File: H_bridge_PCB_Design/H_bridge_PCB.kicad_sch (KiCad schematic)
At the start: 7 parts, among them U1 ESP32-WROOM-32

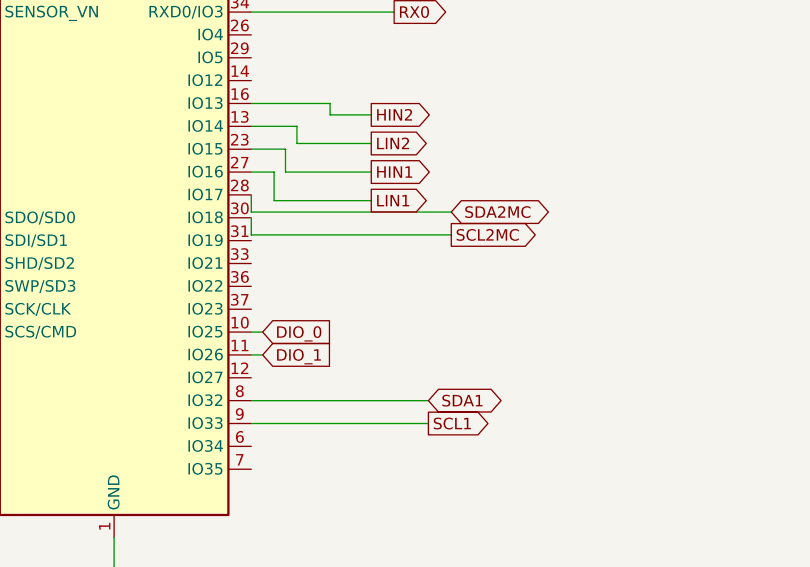
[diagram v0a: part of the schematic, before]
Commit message: huge changes output measurement
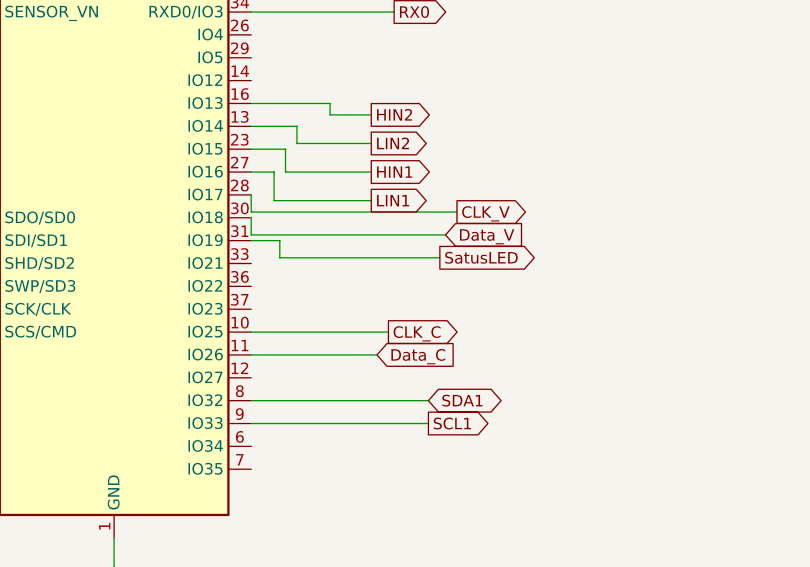
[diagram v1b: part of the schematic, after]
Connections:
- net SatusLED: now reaches U1.31 (IO19)
- net DIO_0 renamed CLK_C
- net DIO_1 renamed Data_C
- net SCL2MC renamed Data_V
- net SDA2MC renamed CLK_V
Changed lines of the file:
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@@
-	(wire
-		(pts
-			(xy 198.12 229.235) (xy 199.39 229.235)
-		)
-		(stroke
-			(width 0)
-			(type default)
-		)
-	)
 	(wire
 		(pts
@@
 	(wire
 		(pts
-			(xy 198.12 213.36) (xy 220.345 213.36)
-		)
-		(stroke
-			(width 0)
-			(type default)
-		)
-	)
-	(wire
-		(pts
 			(xy 201.93 208.915) (xy 211.455 208.915)
 		)
@@
 	(wire
 		(pts
+			(xy 201.295 216.535) (xy 198.12 216.535)
+		)
+		(stroke
+			(width 0)
+			(type default)
+		)
+	)
+	(wire
+		(pts
 			(xy 207.645 179.705) (xy 207.645 183.515)
 		)
@@
 	(wire
 		(pts
-			(xy 198.12 226.695) (xy 199.39 226.695)
-		)
-		(stroke
-			(width 0)
-			(type default)
-		)
-	)
-	(wire
-		(pts
-			(xy 220.345 215.9) (xy 198.12 215.9)
+			(xy 198.12 213.36) (xy 198.12 211.455)
+		)
+		(stroke
+			(width 0)
+			(type default)
+		)
+	)
+	(wire
+		(pts
+			(xy 198.12 213.36) (xy 220.98 213.36)
 		)
 		(stroke
@@
 	(wire
 		(pts
+			(xy 198.12 215.9) (xy 219.71 215.9)
+		)
+		(stroke
+			(width 0)
+			(type default)
+		)
+	)
+	(wire
+		(pts
 			(xy 171.45 163.83) (xy 182.88 163.83)
 		)
@@
 	(wire
 		(pts
-			(xy 198.12 213.36) (xy 198.12 211.455)
+			(xy 213.36 226.695) (xy 198.12 226.695)
 		)
 		(stroke
@@
 	(wire
 		(pts
+			(xy 212.09 229.235) (xy 198.12 229.235)
+		)
+		(stroke
+			(width 0)
+			(type default)
+		)
+	)
+	(wire
+		(pts
 			(xy 201.93 206.375) (xy 198.12 206.375)
 		)
@@
 	(wire
 		(pts
+			(xy 201.295 218.44) (xy 201.295 216.535)
+		)
+		(stroke
+			(width 0)
+			(type default)
+		)
+	)
+	(wire
+		(pts
 			(xy 148.59 175.26) (xy 148.59 183.515)
 		)
@@
 		)
 	)
+	(wire
+		(pts
+			(xy 219.075 218.44) (xy 201.295 218.44)
+		)
+		(stroke
+			(width 0)
+			(type default)
+		)
+	)
 	(global_label "LIN1"
 		(shape output)
@@
 		(property "Intersheetrefs" "${INTERSHEET_REFS}"
 			(at 218.6131 212.09 0)
-			(effects
-				(font
-					(size 1.27 1.27)
-				)
-				(justify left)
-				(hide yes)
-			)
-		)
-	)
-	(global_label "DIO_1"
-		(shape input)
-		(at 199.39 229.235 0)
-		(fields_autoplaced yes)
-		(effects
-			(font
-				(size 1.27 1.27)
-			)
-			(justify left)
-		)
-		(property "Intersheetrefs" "${INTERSHEET_REFS}"
-			(at 207.7576 229.235 0)
 			(effects
 				(font
@@
 		)
 	)
-	(global_label "DIO_0"
-		(shape input)
-		(at 199.39 226.695 0)
-		(fields_autoplaced yes)
-		(effects
-			(font
-				(size 1.27 1.27)
-			)
-			(justify left)
-		)
-		(property "Intersheetrefs" "${INTERSHEET_REFS}"
-			(at 207.7576 226.695 0)
+	(global_label "CLK_V"
+		(shape output)
+		(at 220.98 213.36 0)
+		(fields_autoplaced yes)
+		(effects
+			(font
+				(size 1.27 1.27)
+			)
+			(justify left)
+		)
+		(property "Intersheetrefs" "${INTERSHEET_REFS}"
+			(at 229.5895 213.36 0)
 			(effects
 				(font
@@
 		)
 	)
-	(global_label "SCL2MC"
-		(shape output)
-		(at 220.345 215.9 0)
-		(fields_autoplaced yes)
-		(effects
-			(font
-				(size 1.27 1.27)
-			)
-			(justify left)
-		)
-		(property "Intersheetrefs" "${INTERSHEET_REFS}"
-			(at 230.7687 215.9 0)
-			(effects
-				(font
-					(size 1.27 1.27)
-				)
-				(justify left)
-				(hide yes)
-			)
-		)
-	)
-	(global_label "SDA2MC"
-		(shape bidirectional)
-		(at 220.345 213.36 0)
-		(fields_autoplaced yes)
-		(effects
-			(font
-				(size 1.27 1.27)
-			)
-			(justify left)
-		)
-		(property "Intersheetrefs" "${INTERSHEET_REFS}"
-			(at 231.9405 213.36 0)
-			(effects
-				(font
-					(size 1.27 1.27)
-				)
-				(justify left)
-				(hide yes)
-			)
-		)
-	)
 	(global_label "SCL1"
 		(shape output)
@@
 		)
 	)
+	(global_label "Data_V"
+		(shape input)
+		(at 219.71 215.9 0)
+		(fields_autoplaced yes)
+		(effects
+			(font
+				(size 1.27 1.27)
+			)
+			(justify left)
+		)
+		(property "Intersheetrefs" "${INTERSHEET_REFS}"
+			(at 229.0451 215.9 0)
+			(effects
+				(font
+					(size 1.27 1.27)
+				)
+				(justify left)
+				(hide yes)
+			)
+		)
+	)
 	(global_label "RX0"
 		(shape output)
@@
 		(property "Intersheetrefs" "${INTERSHEET_REFS}"
 			(at 220.6692 191.135 0)
+			(effects
+				(font
+					(size 1.27 1.27)
+				)
+				(justify left)
+				(hide yes)
+			)
+		)
+	)
+	(global_label "Data_C"
+		(shape input)
+		(at 212.09 229.235 0)
+		(fields_autoplaced yes)
+		(effects
+			(font
+				(size 1.27 1.27)
+			)
+			(justify left)
+		)
+		(property "Intersheetrefs" "${INTERSHEET_REFS}"
+			(at 221.6065 229.235 0)
+			(effects
+				(font
+					(size 1.27 1.27)
+				)
+				(justify left)
+				(hide yes)
+			)
+		)
+	)
+	(global_label "CLK_C"
+		(shape output)
+		(at 213.36 226.695 0)
+		(fields_autoplaced yes)
+		(effects
+			(font
+				(size 1.27 1.27)
+			)
+			(justify left)
+		)
+		(property "Intersheetrefs" "${INTERSHEET_REFS}"
+			(at 222.1509 226.695 0)
 			(effects
 				(font
@@
 			(effects
 				(font
+					(size 1.27 1.27)
+				)
+				(justify left)
+				(hide yes)
+			)
+		)
+	)
+	(global_label "SatusLED"
+		(shape output)
+		(at 219.075 218.44 0)
+		(fields_autoplaced yes)
+		(effects
+			(font
+				(size 1.27 1.27)
+			)
+			(justify left)
+		)
+		(property "Intersheetrefs" "${INTERSHEET_REFS}"
+			(at 230.7686 218.44 0)
+			(effects
+				(font

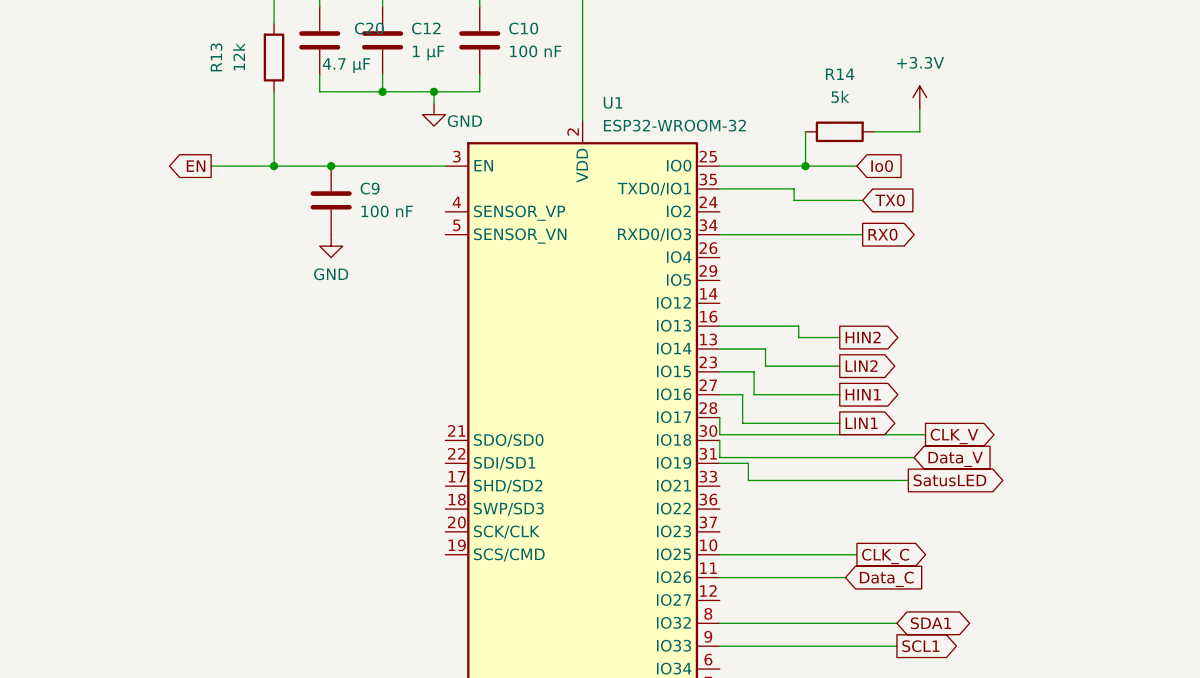
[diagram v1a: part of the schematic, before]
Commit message: new pcb
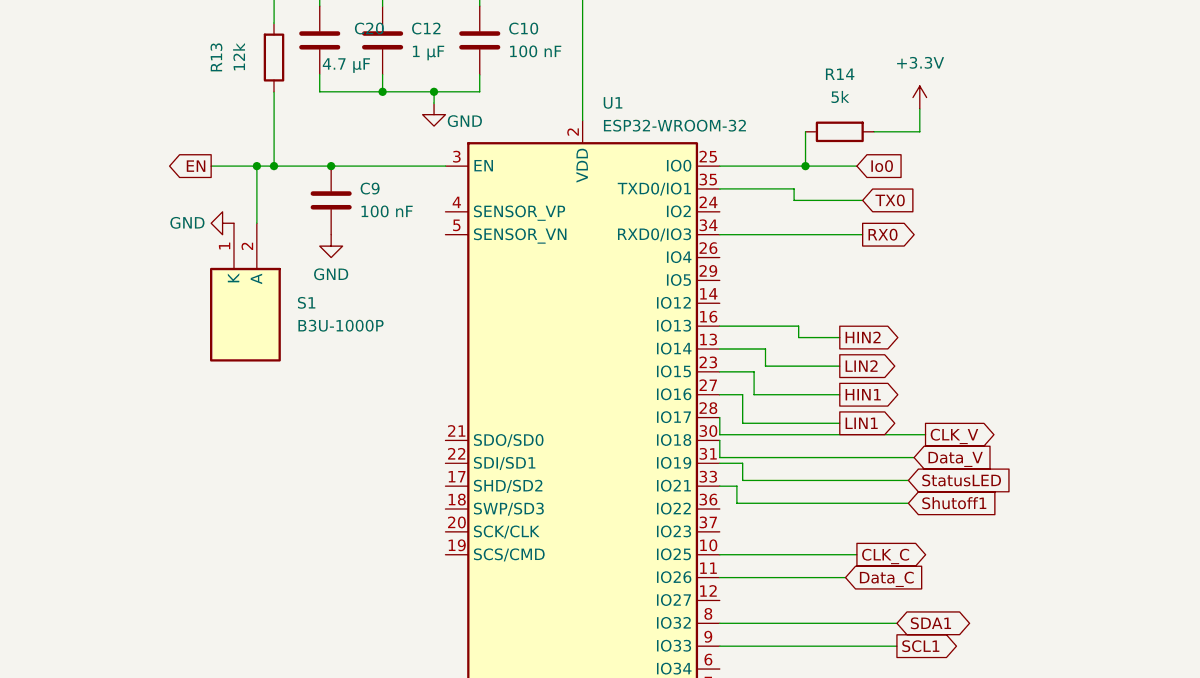
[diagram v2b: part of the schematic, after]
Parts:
- added S1: B3U-1000P, B3U-1000P, symbol SamacSysParts:B3U-1000P
- C10, C20: LCSC Part # (none) -> C49678; LCSC Part# C49678 -> (none)
- C12: LCSC Part # (none) -> C28323; LCSC Part# C28323 -> (none)
- C9: LCSC Part # (none) -> C49678; LCSC Part# C165822 -> (none)
- R13: LCSC Part # (none) -> C139925; LCSC Part# C139925 -> (none)
- R14: LCSC Part # (none) -> C2828700; LCSC Part# C2828700 -> (none)
- U1: LCSC Part # (none) -> C701343; LCSC Part# C701343 -> (none)
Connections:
- net EN: now also S1.2 (A)
- net GND: now also S1.1 (K)
- net Shutoff1: now reaches U1.33 (IO21)
- net SatusLED renamed StatusLED
